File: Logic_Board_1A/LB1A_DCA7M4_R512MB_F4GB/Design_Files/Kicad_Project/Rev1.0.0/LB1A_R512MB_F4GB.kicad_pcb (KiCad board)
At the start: 6 copper layers, 50 x 50 mm, 143 parts, among them U1 STM32MP157CAC3, U2 AS4C256M16D3LC-12BCN, U3 S40FC004C1B2C00000, U4 STPMIC1BPQR, U5 DF40C-70DP-0.4V(51), U6 DF40C-70DP-0.4V(51), U7 DF40C-70DP-0.4V(51), X1 32.768kHz, X2 24MHz

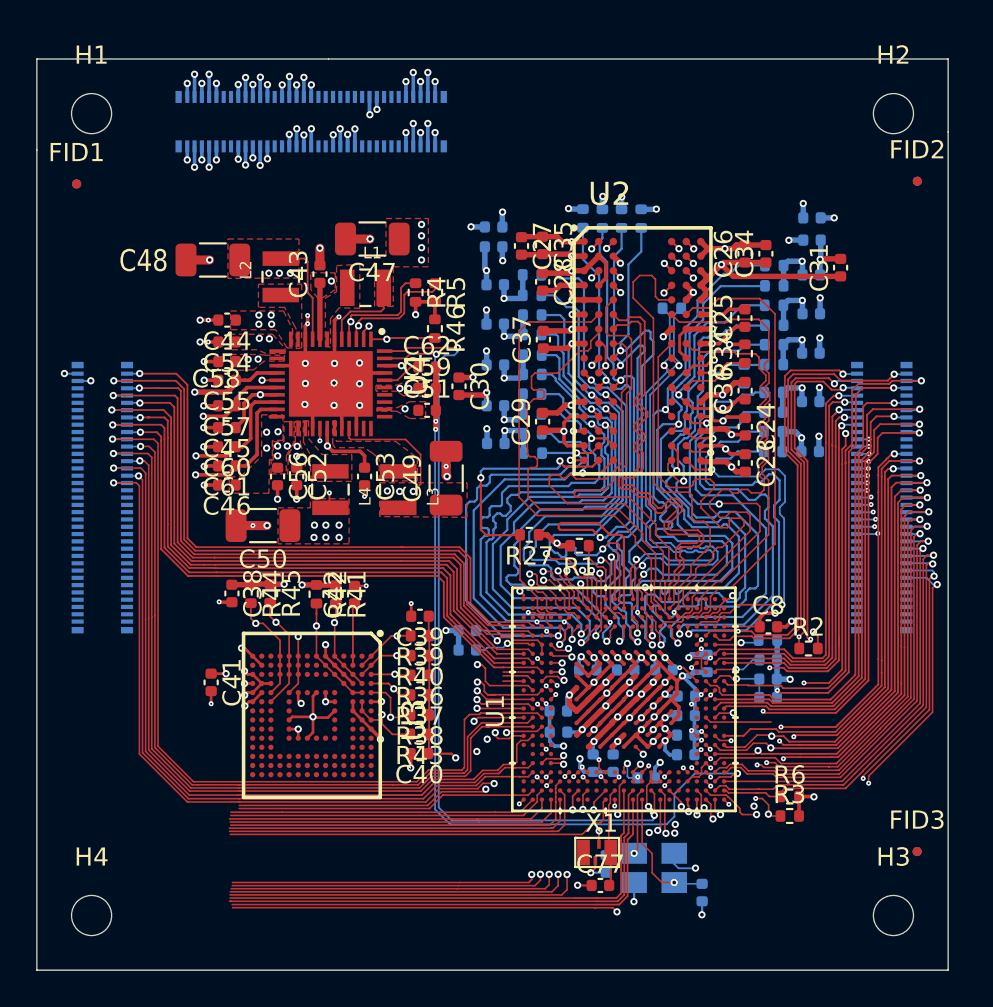
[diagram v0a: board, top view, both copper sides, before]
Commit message: working on connectors
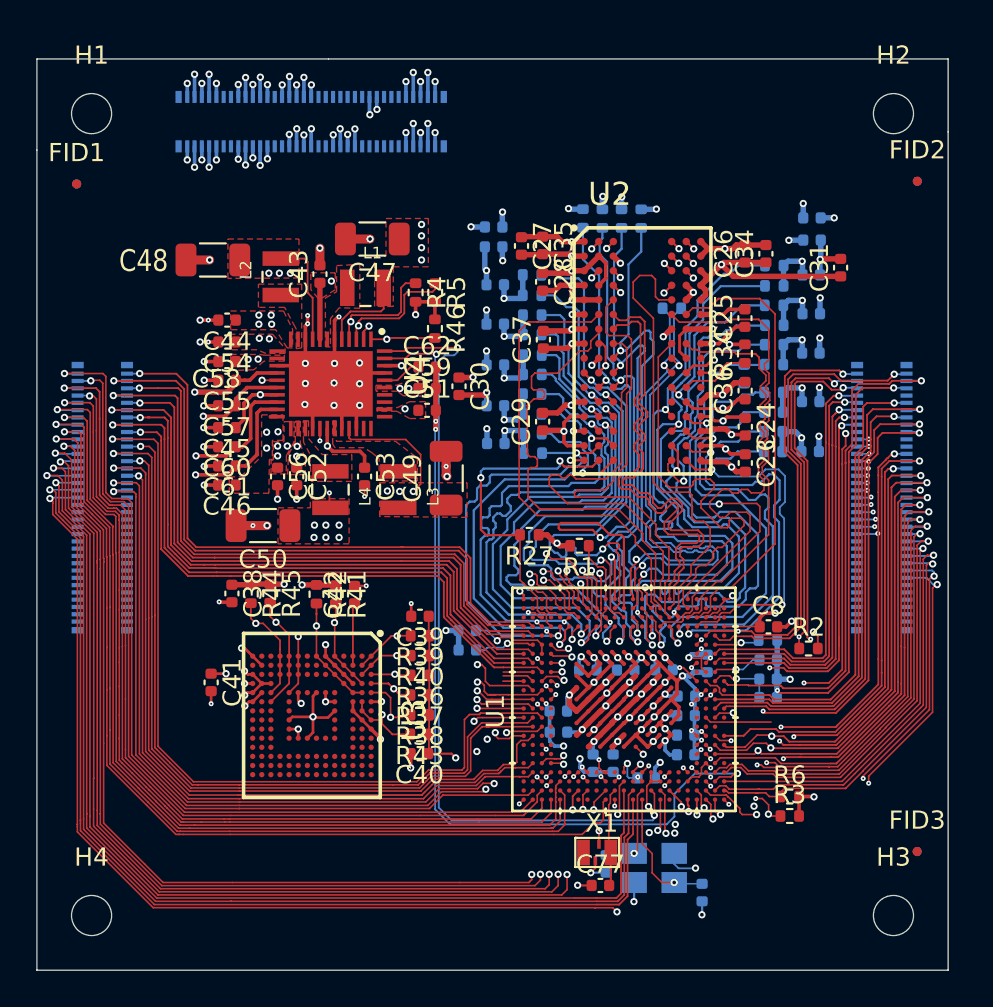
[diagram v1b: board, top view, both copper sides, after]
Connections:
- U5 pad 35: Net-(U5-Pad35) -> BOOT1
- U5 pad 37: Net-(U5-Pad37) -> BOOT0
- U5 pad 38: Net-(U5-Pad38) -> LCD_R7
- U5 pad 39: Net-(U5-Pad39) -> U_BUTTON_1
- U5 pad 41: Net-(U5-Pad41) -> BOOT2
- U5 pad 43: Net-(U5-Pad43) -> LCD_B7
- U5 pad 45: Net-(U5-Pad45) -> LCD_B1
- U5 pad 47: Net-(U5-Pad47) -> LCD_VSYNC
- U5 pad 49: Net-(U5-Pad49) -> USART1_CTS
- U5 pad 51: Net-(U5-Pad51) -> LCD_B6
- U5 pad 53: Net-(U5-Pad53) -> LCD_B0
- U5 pad 55: Net-(U5-Pad55) -> LCD_G7
- U5 pad 57: Net-(U5-Pad57) -> I2S2_SDO
- U5 pad 59: Net-(U5-Pad59) -> LCD_G6
- U5 pad 61: Net-(U5-Pad61) -> LCD_G2
- U5 pad 63: Net-(U5-Pad63) -> LCD_G5
- U5 pad 65: Net-(U5-Pad65) -> LCD_R4
- U5 pad 67: Net-(U5-Pad67) -> LCD_G4
- U5 pad 69: Net-(U5-Pad69) -> LCD_R6
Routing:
- net LCD_B6: track 24.0 -> 56.3 mm, vias 2 -> 3
- net LCD_R6: track 16.5 -> 48.6 mm, vias 0 -> 1
- net BOOT2: track 27.3 -> 59.0 mm, vias 0 -> 1
- net LCD_VSYNC: track 27.3 -> 59.0 mm, vias 2 -> 3
- net LCD_B7: track 27.6 -> 59.0 mm, vias 2 -> 3
- net USART1_CTS: track 24.3 -> 55.5 mm, vias 2 -> 3
- net BOOT0: track 27.3 -> 58.4 mm, vias 0 -> 1
- net LCD_R4: track 17.8 -> 48.7 mm, vias 0 -> 1
- net LCD_B1: track 28.8 -> 59.6 mm, vias 2 -> 3
- net LCD_G6: track 20.1 -> 50.9 mm, vias 0 -> 1
- net BOOT1: track 30.6 -> 61.3 mm, vias 2 -> 3
- net U_BUTTON_1: track 27.7 -> 58.2 mm, vias 0 -> 1
- net LCD_G2: track 18.5 -> 48.7 mm, vias 0 -> 1
- net LCD_G7: track 20.5 -> 50.5 mm, vias 0 -> 1
- net LCD_G4: track 16.9 -> 46.7 mm, vias 0 -> 1
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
